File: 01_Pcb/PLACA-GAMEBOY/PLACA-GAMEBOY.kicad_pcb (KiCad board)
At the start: 2 copper layers, 8 parts, among them J1 Conn_01x08, SW1 SW_Push, SW2 SW_Push, SW3 SW_Push, SW4 SW_Push, SW5 SW_Push, SW6 SW_Push, U1 ESP32-S3-DEVKITC-1-N8R8

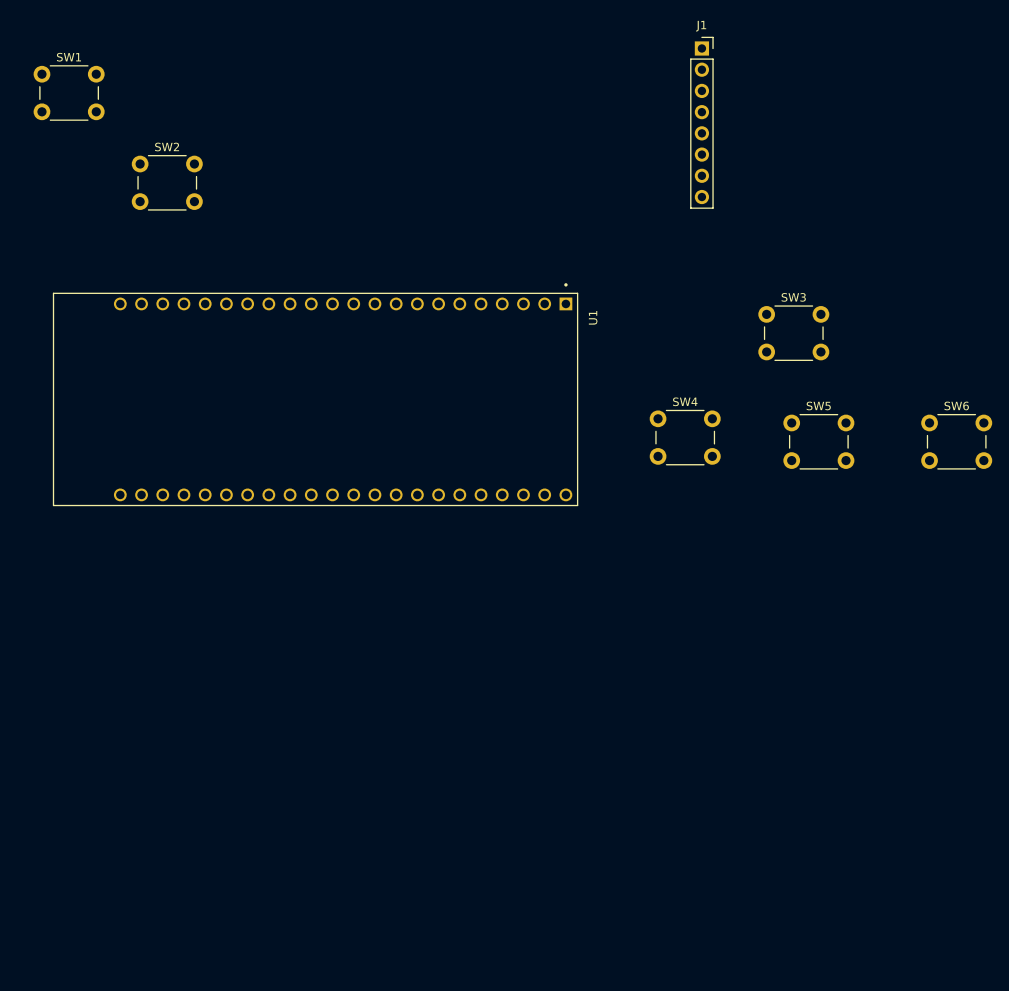
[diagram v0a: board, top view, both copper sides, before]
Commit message: document
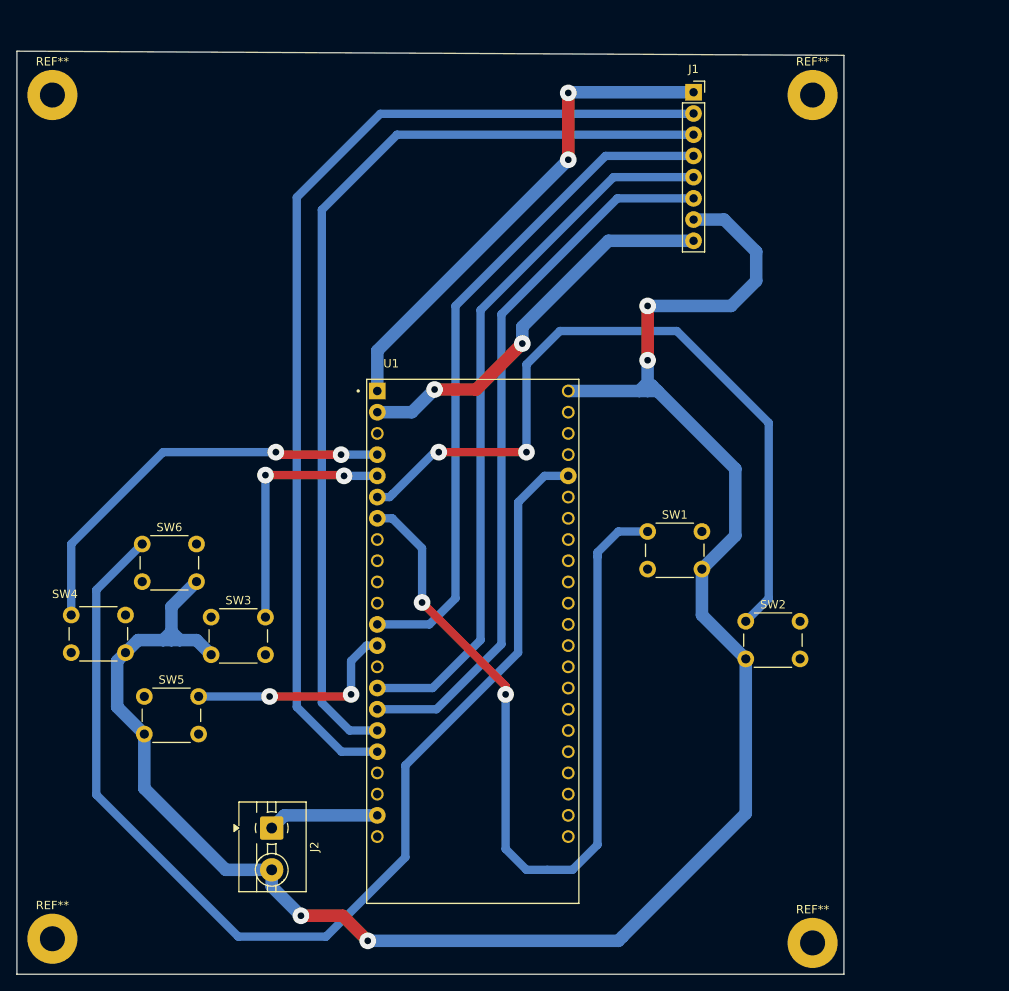
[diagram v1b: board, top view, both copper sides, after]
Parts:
- added J2: Conn_01x02_Socket, TerminalBlock:TerminalBlock_MaiXu_MX126-5.0-02P_1x02_P5.00mm, F.Cu at (73.0, 113.2)
- added REF**: MountingHole_3mm_Pad, MountingHole:MountingHole_3mm_Pad, F.Cu at (137.8, 127.0)
- added REF**: MountingHole_3mm_Pad, MountingHole:MountingHole_3mm_Pad, F.Cu at (46.8, 25.5)
- added REF**: MountingHole_3mm_Pad, MountingHole:MountingHole_3mm_Pad, F.Cu at (46.8, 126.5)
- added REF**: MountingHole_3mm_Pad, MountingHole:MountingHole_3mm_Pad, F.Cu at (137.8, 25.5)
- moved SW6 95.4 mm to (57.5, 79.2)
- moved SW1 90.8 mm to (118.0, 77.7)
- moved SW2 90.8 mm to (129.8, 88.5)
- moved SW5 84.1 mm to (57.8, 97.5)
- moved SW3 75.7 mm to (65.8, 88.0)
- moved SW4 74.1 mm to (49.0, 87.7)
- moved U1 34.5 mm to (97.1, 90.9), turned to 0 degrees
- moved J1 5.33 mm to (123.5, 25.2)
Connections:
- SW3 pad 1: Net-(U1-GPIO4) -> Net-(U1-GPIO5)
- SW4 pad 1: Net-(U1-GPIO5) -> Net-(U1-GPIO4)
- U1 pad J1_21: unconnected-(U1-5V0-PadJ1_21) -> Net-(J2-Pin_1)
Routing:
- net Net-(J1-Pin_7): track 0.00 -> 236.4 mm, vias 0 -> 4
- net Net-(U1-GPIO2): track 0.00 -> 135.7 mm
- net Net-(J1-Pin_2): track 0.00 -> 124.5 mm
- net Net-(J1-Pin_3): track 0.00 -> 115.2 mm
- net Net-(U1-GPIO7): track 0.00 -> 102.3 mm, vias 0 -> 2
- net Net-(U1-GPIO6): track 0.00 -> 90.7 mm, vias 0 -> 2
- net Net-(J1-Pin_5): track 0.00 -> 86.3 mm
- net Net-(J1-Pin_6): track 0.00 -> 86.3 mm
- net Net-(J1-Pin_4): track 0.00 -> 81.6 mm
- net Net-(J1-Pin_1): track 0.00 -> 60.2 mm, vias 0 -> 2
- net Net-(U1-GPIO4): track 0.00 -> 49.8 mm, vias 0 -> 2
- net Net-(J1-Pin_8): track 0.00 -> 47.5 mm, vias 0 -> 2
- net Net-(U1-GPIO5): track 0.00 -> 30.4 mm, vias 0 -> 2
- net Net-(U1-GPIO3): track 0.00 -> 26.3 mm, vias 0 -> 2
- net Net-(J2-Pin_1): track 0.00 -> 13.3 mm
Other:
- board outline added: 99 x 110.5 mm
